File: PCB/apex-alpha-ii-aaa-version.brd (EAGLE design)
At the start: 13.1 x 74.7 mm, 36 parts, among them IC1 CC430F5135, IC2 TPS61200, Y1 26MHz

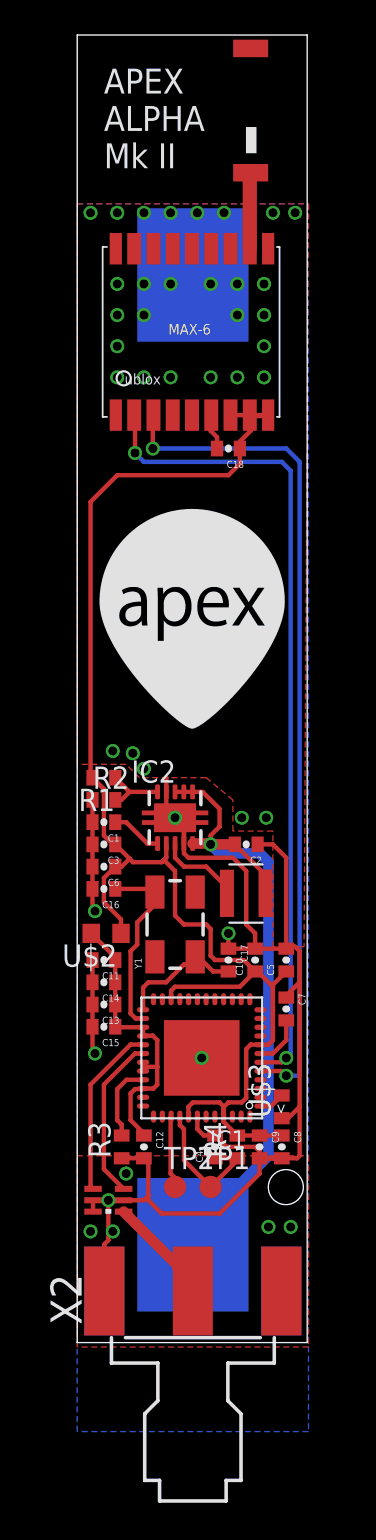
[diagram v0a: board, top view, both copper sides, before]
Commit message: New PCB layout etc.
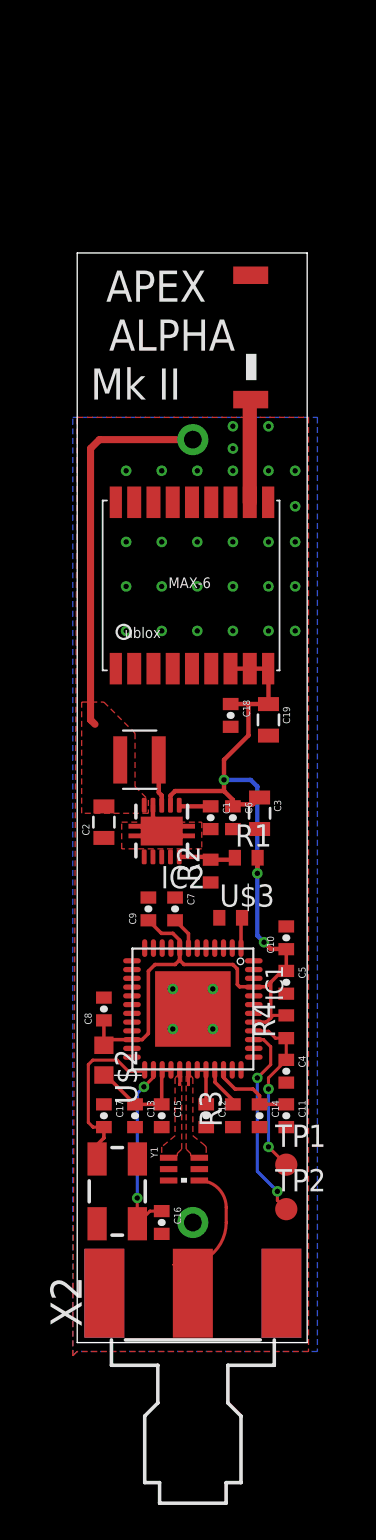
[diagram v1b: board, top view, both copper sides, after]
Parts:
- removed U$4: (no value), !danielparts:APEXHAB-LOGO-SMALL
- added C19: 4.7uF, apex:0805
- AAA: device apex:SMD-BATTERY-HOLDER-AAA -> apex:THROUGH-HOLE-BATTERY-HOLDER-AAA
- C10: value 10uF -> 1uF
- C2, C3: device apex:0402-CAP -> apex:0805
- C9: value 10uF -> 100nF
- moved C16 19.3 mm to (4.83, 6.86), turned to 270 degrees
- moved Y1 15.6 mm to (2.29, 8.64), turned to 270 degrees
- moved C18 15.2 mm to (8.76, 35.8), turned to 270 degrees
- moved C9 15.0 mm to (4.06, 24.8), turned to 90 degrees
- moved GPS 14.5 mm to (6.60, 43.4)
- moved C11 13.7 mm to (11.9, 13.0), turned to 270 degrees
- moved U$1 13.0 mm to (8.64, 57.7)
- moved C8 12.9 mm to (1.52, 19.1), turned to 90 degrees
- moved C14 11.7 mm to (10.4, 13.0), turned to 270 degrees
- moved C17 11.4 mm to (1.52, 13.0)
- moved U$3 11.2 mm to (8.76, 24.3), turned to 0 degrees
- moved NR3015 9.76 mm to (3.56, 33.3), turned to 180 degrees
- moved R1 9.33 mm to (9.65, 27.7), turned to 0 degrees
- moved C3 9.07 mm to (10.4, 30.2), turned to 270 degrees
- moved C7 8.54 mm to (5.59, 24.8)
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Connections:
- net GND: now also C19.2
- net VCC: now also C19.1
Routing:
- net GND: track 89.7 -> 1.41 mm, vias 42 -> 32
- net GPSRX: track 48.0 -> 0.00 mm, vias 2 -> 0
- net GPSTX: track 46.7 -> 0.00 mm, vias 2 -> 0
- net VCC: track 81.1 -> 58.7 mm, vias 0 -> 3
- net N$1: track 38.5 -> 21.9 mm, vias 1 -> 0
- net N$6: track 10.2 -> 0.85 mm
- net N$2: track 9.40 -> 0.84 mm
- net N$12: track 4.13 -> 11.4 mm, vias 0 -> 2
- net VEE: track 17.5 -> 13.9 mm
- net N$13: track 7.21 -> 9.90 mm
- net N$7: track 6.63 -> 9.18 mm
- net N$3: track 4.81 -> 2.66 mm
- net N$9: track 4.45 -> 2.40 mm
- net N$11: track 8.28 -> 10.1 mm, vias 0 -> 2
- net N$8: track 4.36 -> 5.89 mm
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- added copper zone on layer 1, net N$1
- added copper zone on layer 1, net N$2
- added copper zone on layer 1, net N$6
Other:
- board size 13.1 x 74.7 mm -> 13.1 x 62.2 mm
- board text added: "ALPHA"
- board text added: "APEX"
- board text added: "Mk II"
- board text removed: ">"
- board text removed: "APEX ALPHA Mk II"
- board text removed: "DANIEL"
- board text removed: "Dec 2012"
- board text removed: "SAUL"
- board text removed: "You need to put a battery here."
